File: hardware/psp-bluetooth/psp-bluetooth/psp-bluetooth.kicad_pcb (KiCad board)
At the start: 2 copper layers, 58.4 x 85.1 mm, 16 parts, among them J1 Left Connector, J2 Center Connector, J3 Right Connector, J4 Analog Connector, J5 PSP Power out, J6 Power IN, J7 Serial, J8 Vin Toggle, P1 Digital, P2 Analog, P3 CONN_01X01, P4 CONN_01X01, P5 CONN_01X01, P6 CONN_01X01, U1 MCP4251-xxxx-P

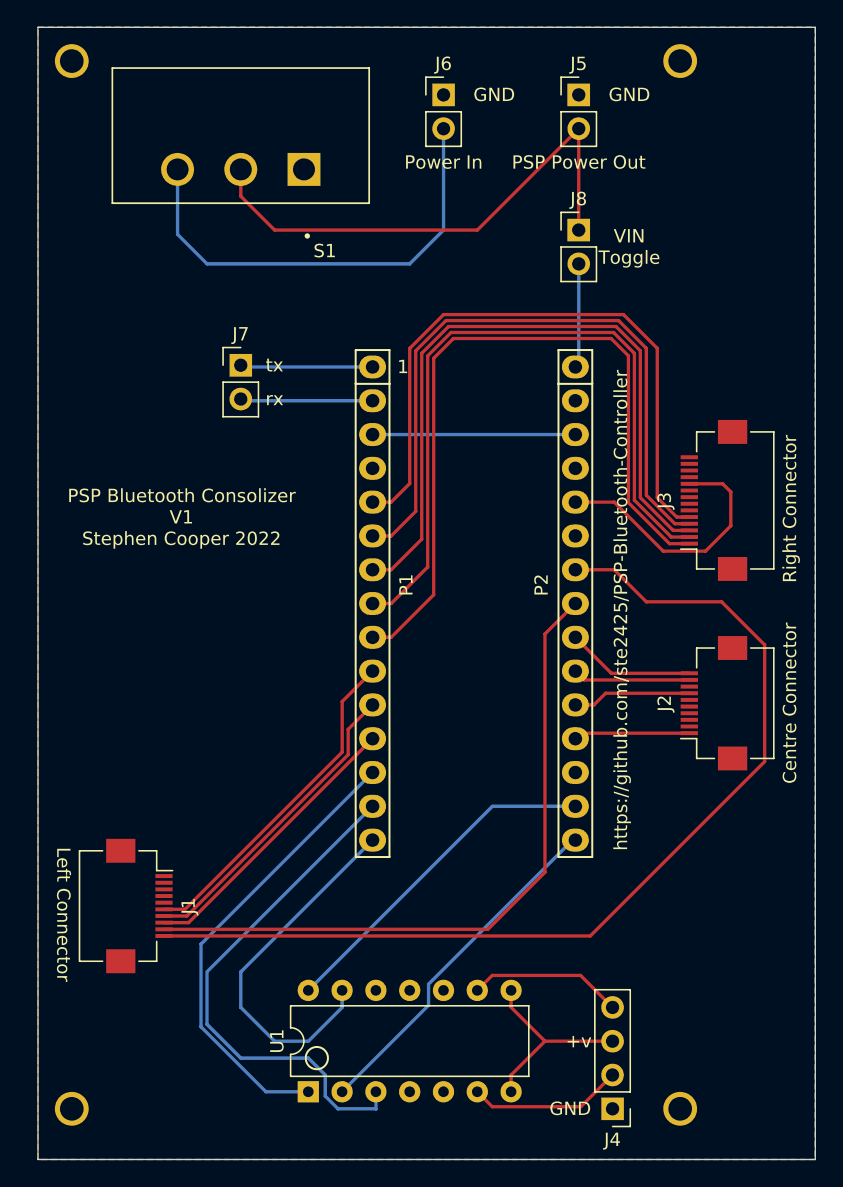
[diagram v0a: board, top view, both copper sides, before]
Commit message: Initial work and hardware stuff
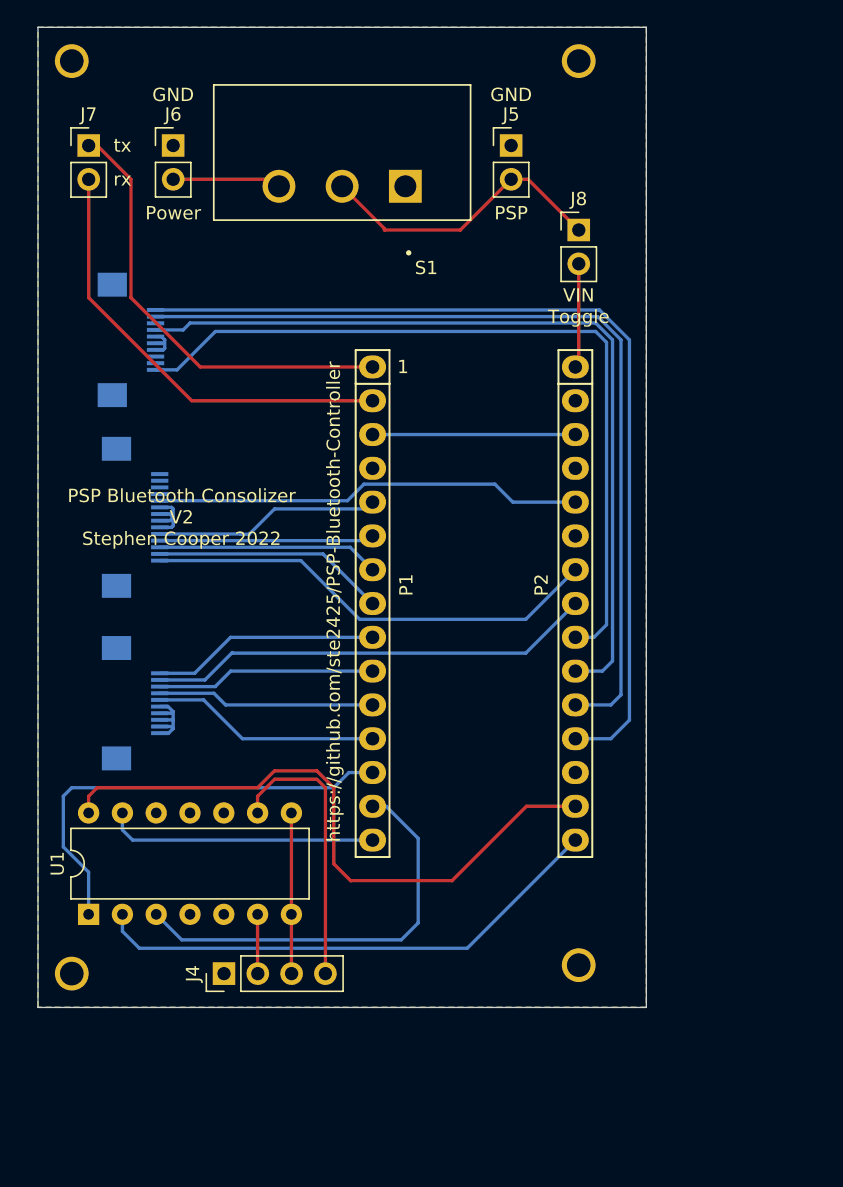
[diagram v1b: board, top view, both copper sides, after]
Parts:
- J1, J2, J3: moved to B.Cu
- moved J2 51.6 mm to (121.3, 69.2)
- moved J3 43.5 mm to (121.6, 82.5)
- moved J4 30.9 mm to (128.3, 116.8), turned to 90 degrees
- moved U1 21.2 mm to (118.1, 112.4)
- moved J6 20.7 mm to (124.5, 54.6)
- moved J7 20.1 mm to (118.1, 54.6)
- moved J1 15.2 mm to (121.6, 96.5), turned to 90 degrees
- moved P5 13.2 mm to (154.9, 116.2)
- moved P4 10.2 mm to (116.8, 116.8)
- moved S1 7.73 mm to (137.2, 57.7)
- moved P6 7.62 mm to (154.9, 48.3)
- moved J5 6.35 mm to (149.9, 54.6)
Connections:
- J1 pad 10: /A5 (D19) -> /6(**)
- J1 pad 6: /7 -> /9(**)
- J1 pad 8: /9(**) -> /7
- J2 pad 1: /A0 (D14) -> /A3 (D17)
- J2 pad 10: /A3 (D17) -> /A0 (D14)
- J2 pad 7: /A1 (D15) -> /A2 (D16)
- J2 pad 9: /A2 (D16) -> /A1 (D15)
- J3 pad 1: /6(**) -> /A5 (D19)
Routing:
- net /A0 (D14): track 8.74 -> 69.8 mm
- net /A1 (D15): track 8.93 -> 66.1 mm
- net /A2 (D16): track 8.84 -> 62.3 mm
- net /A3 (D17): track 9.68 -> 59.4 mm
- net /A5 (D19): track 75.9 -> 34.6 mm
- net /6(**): track 56.4 -> 17.1 mm
- net /5(**): track 54.4 -> 17.5 mm
- net /4: track 52.4 -> 16.7 mm
- net /3(**): track 50.4 -> 16.1 mm
- net /2: track 48.5 -> 17.0 mm
- net Net-(J6-Pad2): track 34.5 -> 8.17 mm
- net /1(Tx): track 9.96 -> 33.4 mm
- net /0(Rx): track 9.96 -> 33.4 mm
- net +3V3: track 25.8 -> 47.7 mm
- net /A4 (D18): track 51.5 -> 33.7 mm
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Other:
- board size 58.4 x 85.1 mm -> 45.7 x 73.7 mm
- board text added: "PSP"
- board text added: "PSP Bluetooth Consolizer V2 Stephen Cooper 2022"
- board text added: "Power"
- board text removed: "+v"
- board text removed: "Centre Connector"
- board text removed: "Left Connector"
- board text removed: "PSP Bluetooth Consolizer V1 Stephen Cooper 2022"
- board text removed: "PSP Power Out"
- board text removed: "Power In"
- board text removed: "Right Connector"
